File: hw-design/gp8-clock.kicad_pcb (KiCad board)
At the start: 2 copper layers, 90 x 36 mm, 82 parts, among them P1 CONN_01X03, Q1 Q_NPN_BCE, Q2 Q_NPN_BCE, SW1 SW_PUSH, SW2 power, U1 TSOP39538, U2 weight-scale-lcd, U3 STM32F0-LQFP48, U4 usb-micro, U5 MCP73833, U6 AP1117D33, U7 nRF8001, Y1 Crystal, Y2 32kHz, Y3 16MHz

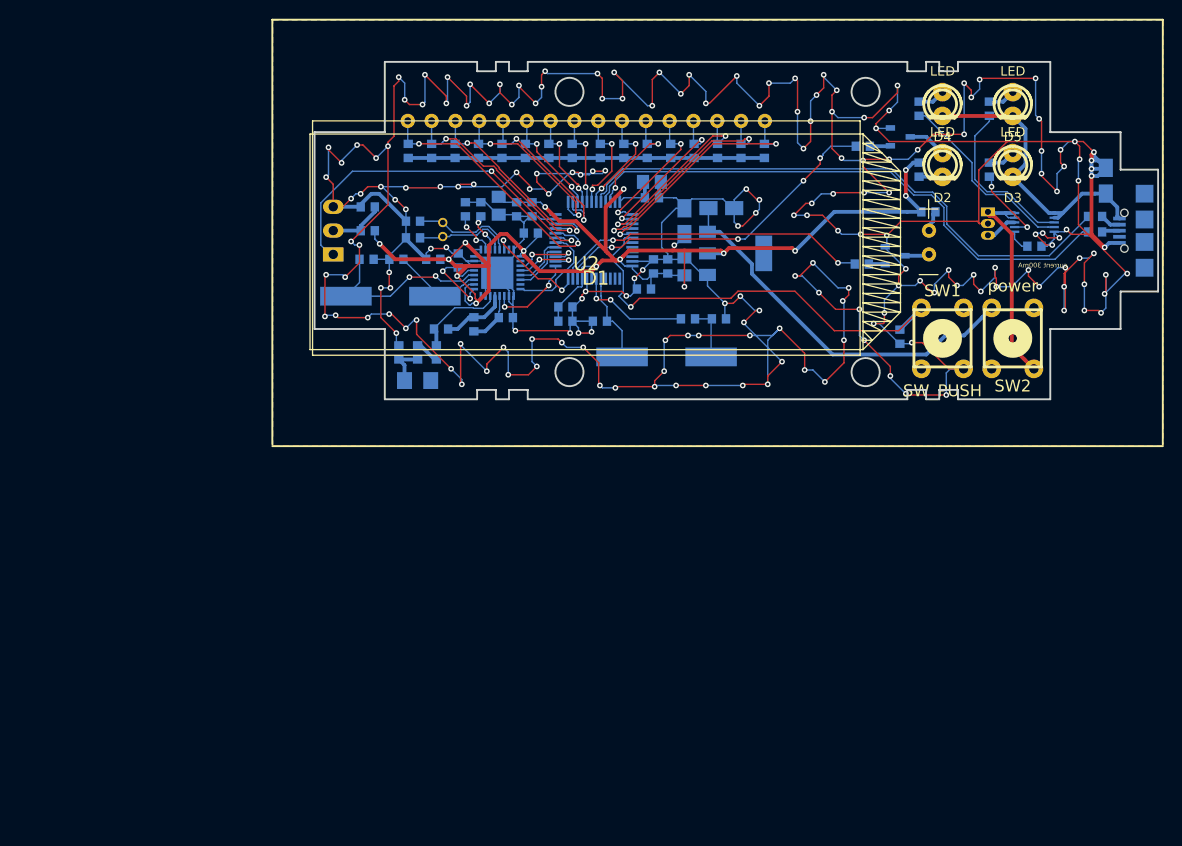
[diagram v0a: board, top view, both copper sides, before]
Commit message: Powiększona płytka
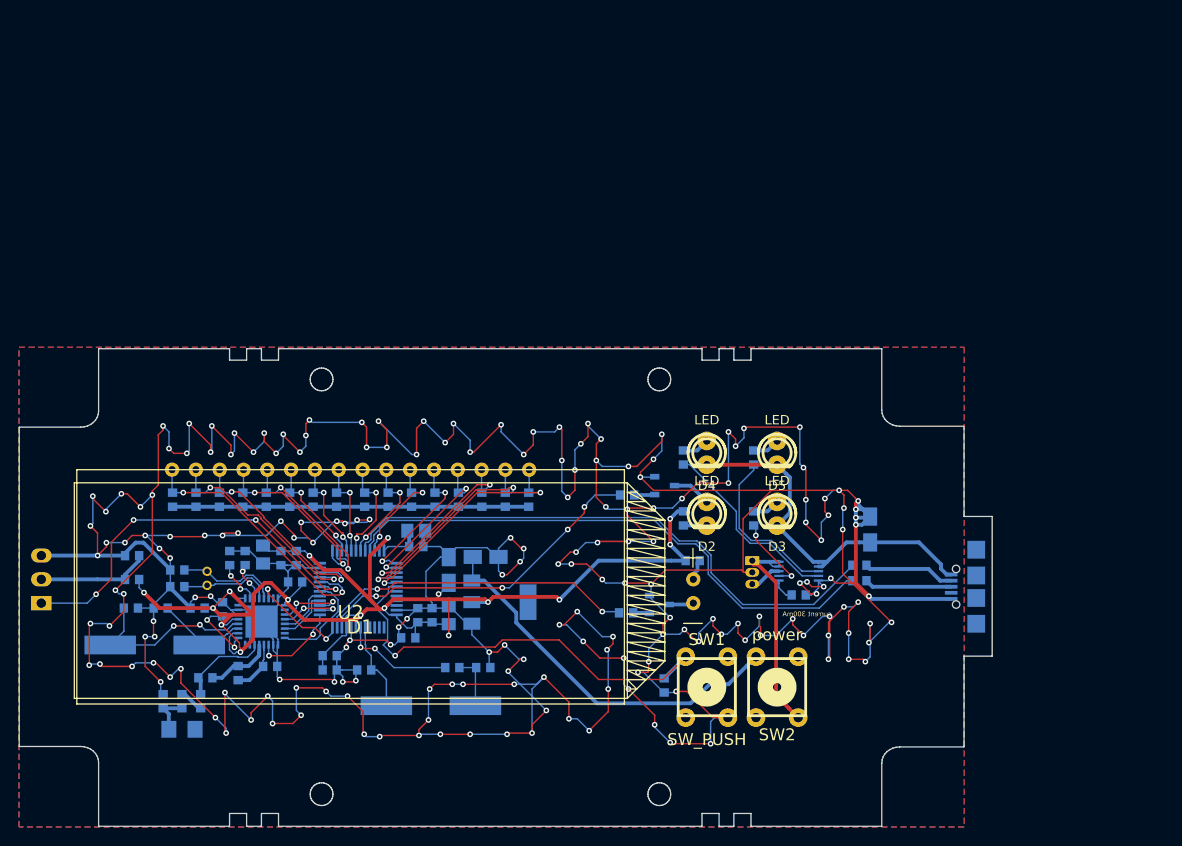
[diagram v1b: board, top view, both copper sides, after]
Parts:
- moved U1 48.5 mm to (103.9, 101.7)
- moved C11 44.9 mm to (147.3, 105.5)
- moved C20 44.9 mm to (124.0, 99.4)
- moved C23 44.9 mm to (120.5, 104.8)
- moved C25 44.9 mm to (116.6, 104.8)
- moved C8 44.9 mm to (131.1, 99.4)
- moved R23 44.9 mm to (191.1, 100.2)
- moved C12 44.9 mm to (170.3, 113.0)
- moved C15 44.9 mm to (192.3, 96.4)
- moved C17 44.9 mm to (147.3, 100.7)
- moved C21 44.9 mm to (125.6, 99.4)
- moved C3 44.9 mm to (138.3, 111.4)
- moved C4 44.9 mm to (151.0, 111.1)
- moved C6 44.9 mm to (127.5, 99.1)
- moved R22 44.9 mm to (147.7, 111.1)
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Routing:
- net GND: track 798.5 -> 811.8 mm, vias 195 -> 196
- net Net-(R24-Pad1): track 1.90 -> 9.49 mm
- net Net-(R23-Pad1): track 2.21 -> 9.75 mm
- net +5V: track 31.9 -> 39.2 mm
- net Net-(C1-Pad1): track 6.10 -> 12.1 mm
- net /ir: track 39.2 -> 42.3 mm, vias 2 -> 4
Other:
- board size 90 x 36 mm -> 103.8 x 50.9 mm
